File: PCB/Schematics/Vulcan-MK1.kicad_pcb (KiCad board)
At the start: 4 copper layers, 108.5 x 93 mm, 146 parts, among them J1 USB_C_Receptacle_USB2.0_16P, J14 Conn_01x02, J15 Power_In, J16 Conn_01x05, J17 Conn_01x02, J18 Conn_01x02, J19 Conn_01x02, J20 Conn_01x03, J21 EXP1, J22 EXP2, J23 5015_Connector, J24 3010_Connector, J25 Conn_01x02, J26 Conn_01x02, J27 Conn_01x04, J28 Conn_01x04, J29 Conn_01x04, J30 Conn_01x03, J31 Conn_01x03, J32 Conn_01x04, J33 Conn_01x04, J34 Conn_01x03, J35 Conn_01x03, J36 Conn_01x03, J37 Conn_01x03, J8 Micro_SD_Card_Det1, Q1 IRF4905, Q2 IRLB8721PBF, Q3 IRLB8721PBF, SW1 SW_Push, SW3 SW_SPDT, U1 STM32F407VETx, U2 TMC2209_SILENTSTEPSTICK, U3 TMC2209_SILENTSTEPSTICK, U4 TMC2209_SILENTSTEPSTICK, U5 TMC2209_SILENTSTEPSTICK, U6 TMC2209_SILENTSTEPSTICK, U8 AMS1117-3.3, U9 TPS54202DDC, Y1 8MHz

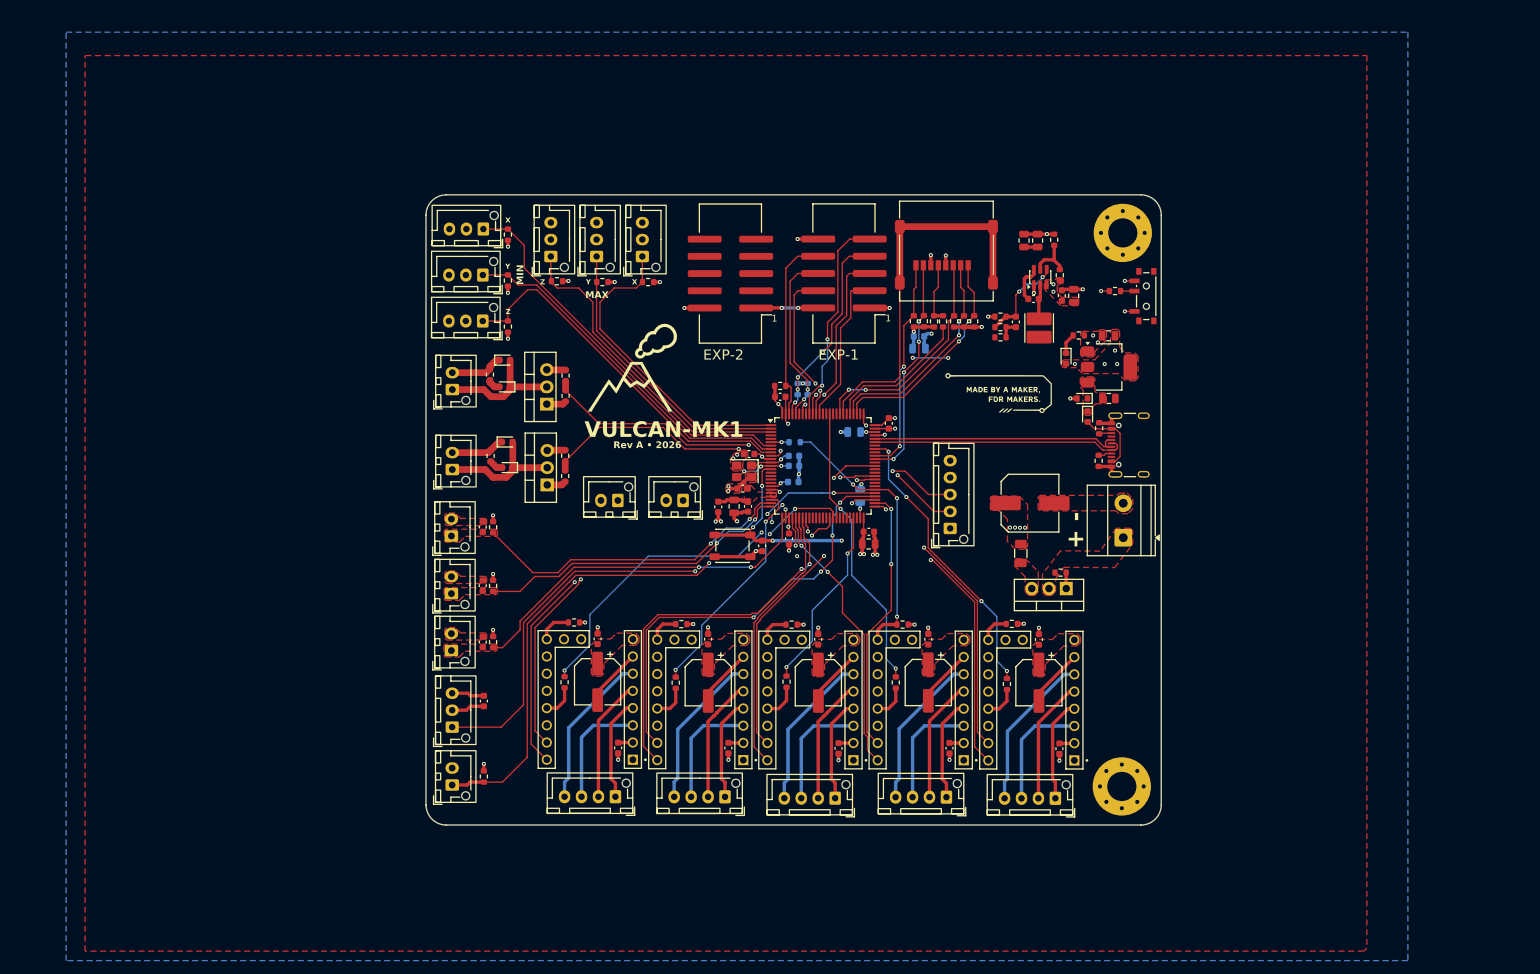
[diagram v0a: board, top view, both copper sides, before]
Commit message: Add changes
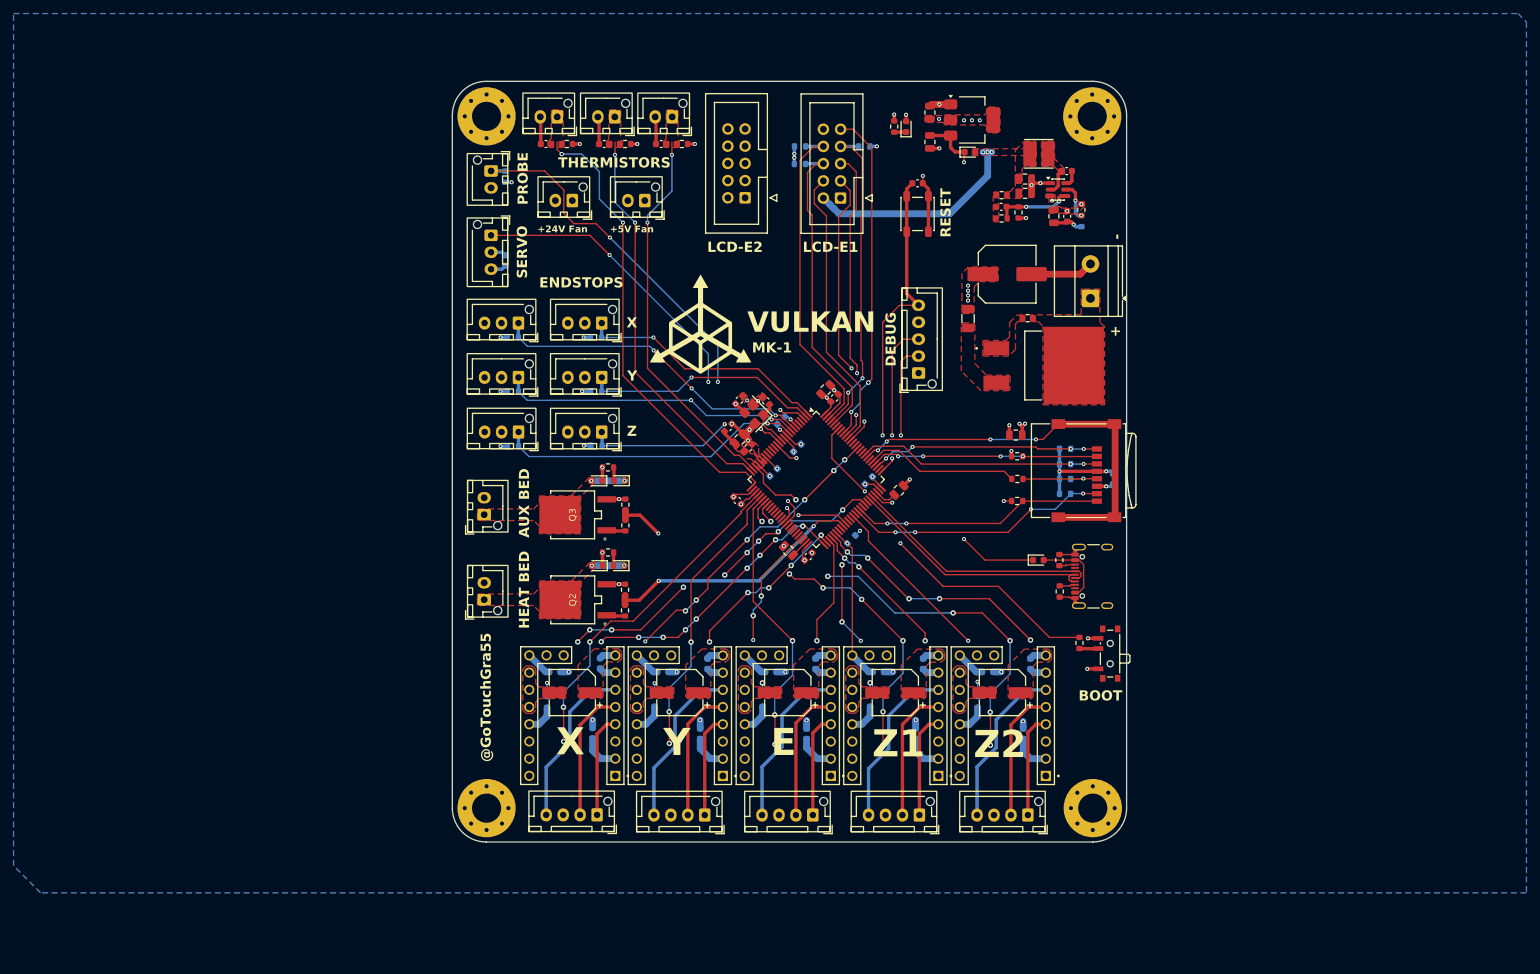
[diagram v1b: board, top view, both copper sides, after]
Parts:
- removed .: LOGO, LOGO
- removed C37, C39: 100nF, Capacitor_SMD:C_0603_1608Metric
- removed C38: 10uF, Capacitor_SMD:C_0805_2012Metric
- removed C40, C41: 22uF, Capacitor_SMD:C_0805_2012Metric
- removed C42: 75pF, Capacitor_SMD:C_0603_1608Metric
- removed the G*** at (174.5, 86.2)
- removed R29: 511K, Resistor_SMD:R_0603_1608Metric
- removed R30: 105K, Resistor_SMD:R_0603_1608Metric
- removed R31: 49.9R, Resistor_SMD:R_0603_1608Metric
- removed R32: 100K, Resistor_SMD:R_0603_1608Metric
- removed R33: 13.3K, Resistor_SMD:R_0603_1608Metric
- removed the REF** at (198.9, 62.6)
- removed the REF** at (198.8, 144.3)
- removed U9: TPS54202DDC, Package_TO_SOT_SMD:SOT-23-6
- added C12: 100nF, Capacitor_SMD:C_0603_1608Metric, F.Cu at (190.7, 60.2)
- added C17: 10uF, Capacitor_SMD:C_0805_2012Metric, F.Cu at (188.8, 60.2)
- added C18: 100nF, Capacitor_SMD:C_0603_1608Metric, F.Cu at (190.7, 53.5)
- added C19: 22uF, Capacitor_SMD:C_0805_2012Metric, F.Cu at (184.5, 54.7)
- added C20: 22uF, Capacitor_SMD:C_0805_2012Metric, F.Cu at (184.5, 56.8)
- added C21: 75pF, Capacitor_SMD:C_0603_1608Metric, F.Cu at (181.0, 58.8)
- added G***: LOGO, Vulkan:Vulkan, F.Cu at (136.6, 76.1)
- added R4: 511K, Resistor_SMD:R_0603_1608Metric, F.Cu at (192.8, 59.2)
- added R5: 105K, Resistor_SMD:R_0603_1608Metric, B.Cu at (192.8, 60.9)
- added R6: 49.9R, Resistor_SMD:R_0603_1608Metric, F.Cu at (181.1, 57.0)
- added R7: 100K, Resistor_SMD:R_0603_1608Metric, F.Cu at (181.1, 60.5)
- added R8: 13.3K, Resistor_SMD:R_0603_1608Metric, F.Cu at (183.6, 59.6)
- added REF**: MountingHole_4.3mm_M4_Pad_Via, MountingHole:MountingHole_4.3mm_M4_Pad_Via, F.Cu at (194.5, 147.5)
- added REF**: MountingHole_4.3mm_M4_Pad_Via, MountingHole:MountingHole_4.3mm_M4_Pad_Via, F.Cu at (194.4, 45.4)
- added REF**: MountingHole_4.3mm_M4_Pad_Via, MountingHole:MountingHole_4.3mm_M4_Pad_Via, F.Cu at (105.0, 45.4)
- added REF**: MountingHole_4.3mm_M4_Pad_Via, MountingHole:MountingHole_4.3mm_M4_Pad_Via, F.Cu at (105.0, 147.5)
- added U7: TPS54202DDC, Package_TO_SOT_SMD:SOT-23-6, F.Cu at (189.4, 56.2)
- C1, C29, C30, C46, C5, C50, C52, C53, C54, C56, C58, C59, C61, FB1, R17, R18, R19, R21, R37, R39, R48, R49, R50, R51, R52, R53, R54, R55, R56, R57, R58, R59, R60, R61, R62, R63: moved to B.Cu
- C15, C16, C35, C8, C9: moved to F.Cu
- J21, J22: footprint Connector_IDC:IDC-Header_2x05_P2.54mm_Vertical_SMD -> Connector_IDC:IDC-Header_2x05_P2.54mm_Vertical
- J8: footprint SDSocket:microSD_HC_Molex_47219 -> Connector_Card:microSD_HC_Wuerth_693072010801
- Q1: footprint Package_TO_SOT_THT:TO-220-3_Vertical -> IRF4905STRLPBF:TRANS_IRF3205S
- Q2, Q3: footprint Package_TO_SOT_THT:TO-220-3_Vertical -> AOD4184A:TO252_AOS
- moved J19 90.8 mm to (105.7, 53.5), turned to -90 degrees
- moved R37 88.6 mm to (107.8, 54.3), turned to 90 degrees
- moved J18 80.3 mm to (115.5, 45.5), turned to 180 degrees
- moved J17 74.4 mm to (124.0, 45.5), turned to 180 degrees
- moved R36 74.3 mm to (116.9, 49.5), turned to 180 degrees
- moved C45 74.1 mm to (113.8, 49.5), turned to 180 degrees
- moved J20 72.8 mm to (105.7, 63.0), turned to -90 degrees
- moved J14 69.9 mm to (132.4, 45.5), turned to 180 degrees
- moved C29 68.9 mm to (120.7, 136.4), turned to -90 degrees
- moved C31 68.9 mm to (117.7, 130.4), turned to 180 degrees
- moved R35 68.1 mm to (125.5, 49.5), turned to 180 degrees
- moved R51 67.9 mm to (114.0, 131.8)
- moved R48 67.8 mm to (115.1, 127.4)
- moved U2 67.8 mm to (117.7, 133.8)
- moved J27 67.7 mm to (121.4, 148.5)
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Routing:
- net +5V: track 17.0 -> 95.9 mm
- net Net-(D1-K): track 0.00 -> 75.8 mm, vias 0 -> 2
- net MOTOR_Z2: track 62.4 -> 34.2 mm, vias 5 -> 2
- net GND: track 128.0 -> 101.9 mm, vias 34 -> 27
- net DRIVER_EN: track 128.8 -> 107.3 mm, vias 3 -> 1
- net BTN_ENC: track 27.8 -> 48.7 mm
- net BTN_EN1: track 26.0 -> 46.5 mm, vias 2 -> 0
- net M4_STEP: track 63.5 -> 43.3 mm, vias 4 -> 3
- net M1_STEP: track 42.5 -> 62.8 mm, vias 2 -> 9
- net LCD_CS: track 22.8 -> 42.0 mm, vias 0 -> 2
- net M5_STEP: track 76.3 -> 57.5 mm, vias 3 -> 5
- net LCD_SCK: track 23.4 -> 42.0 mm, vias 2 -> 0
- net MOTOR_X: track 42.9 -> 61.3 mm, vias 4 -> 10
- net BEEPER: track 31.4 -> 49.6 mm, vias 2 -> 3
- net BTN_EN2: track 29.7 -> 47.5 mm, vias 4 -> 2
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- added copper zone on In1.Cu, net +3.3V
- added copper zone on In2.Cu, net GND
- added copper zone on F.Cu, net Net-(C21-Pad1)
- added copper zone on F.Cu, net Net-(D3-A)
- added copper zone on F.Cu, net Net-(D5-K)
- added copper zone on F.Cu, net Net-(Q1-G)
- added copper zone on F.Cu, net Net-(U7-SW)
- removed copper zone on In2.Cu, net +3.3V
- removed copper zone on In1.Cu, net GND
- removed copper zone on F.Cu, net Net-(D1-K)
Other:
- board size 108.5 x 93 mm -> 99.5 x 112.2 mm
- board text added: "+"
- board text added: "+24V Fan"
- board text added: "+5V Fan"
- board text added: "-"
- board text added: "@GoTouchGra55"
- board text added: "AUX BED"
- board text added: "BOOT"
- board text added: "DEBUG"
- board text added: "E"
- board text added: "ENDSTOPS"
- board text added: "HEAT BED"
- board text added: "INPUT"
- board text added: "LCD-E1"
- board text added: "LCD-E2"
- board text added: "MK-1"
- board text added: "PROBE"
- board text added: "RESET"
- board text added: "SERVO"
- board text added: "SWCLK"
- board text added: "SWDIO"
- board text added: "THERMISTORS"
- board text added: "VULKAN"
- board text added: "Z1"
- board text added: "Z2"
- board text removed: "+ -"
- board text removed: "1"
- board text removed: "AUX THR"
- board text removed: "BED THR"
- board text removed: "CLK"
- board text removed: "D"
- board text removed: "DIO"
- board text removed: "EXP-1"
- board text removed: "EXP-2"
- board text removed: "Ex-Stepper"
- board text removed: "G"
- board text removed: "HOTEND"
- board text removed: "M1A1"
- board text removed: "M1A2"
- board text removed: "M1A3"
- board text removed: "M1A4"
- board text removed: "M1A5"
- board text removed: "M1B1"
- board text removed: "M1B2"
- board text removed: "M1B3"
- board text removed: "M1B4"
- board text removed: "M1B5"
- board text removed: "M2A1"
- board text removed: "M2A2"
- board text removed: "M2A3"
- board text removed: "M2A4"
- board text removed: "M2A5"
- board text removed: "M2B1"
- board text removed: "M2B2"
- board text removed: "M2B3"
- board text removed: "M2B4"
- board text removed: "M2B5"
- board text removed: "Rev A • 2026"
- board text removed: "S"
- board text removed: "VULCAN-MK1"
- board text removed: "X-Stepper"
- board text removed: "Y-Stepper"
- board text removed: "Z1-Stepper"
- board text removed: "Z2-Stepper"
- board text removed: "© 2026 Shaurya Tamang MIT License github.com/GoTouchGra55/NOT-618"
